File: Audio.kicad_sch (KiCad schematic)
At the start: 21 parts, among them CN2 PJ-3537S, U3 SGTL5000XNAA3R2, U8 PCM1807PW, X1 SMD-3225_4P 12.288MHZ 12PF

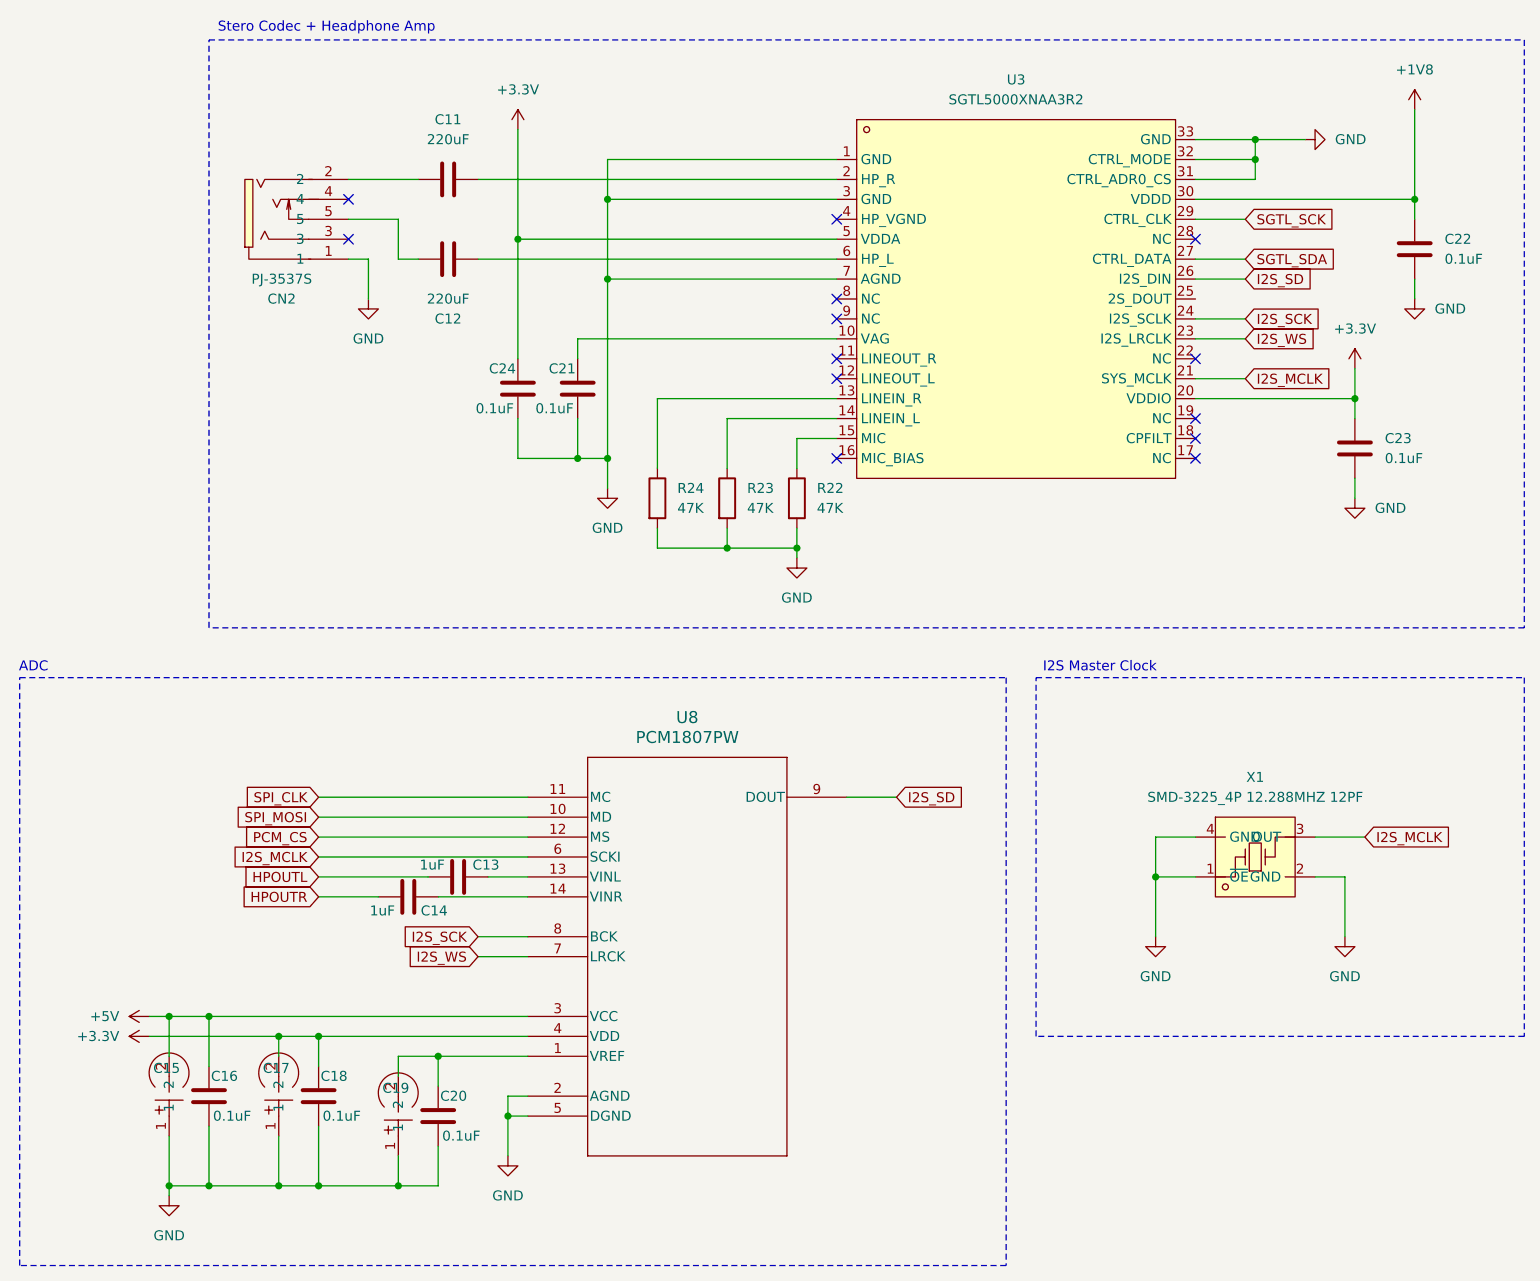
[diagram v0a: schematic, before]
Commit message: start of adding esp32 module
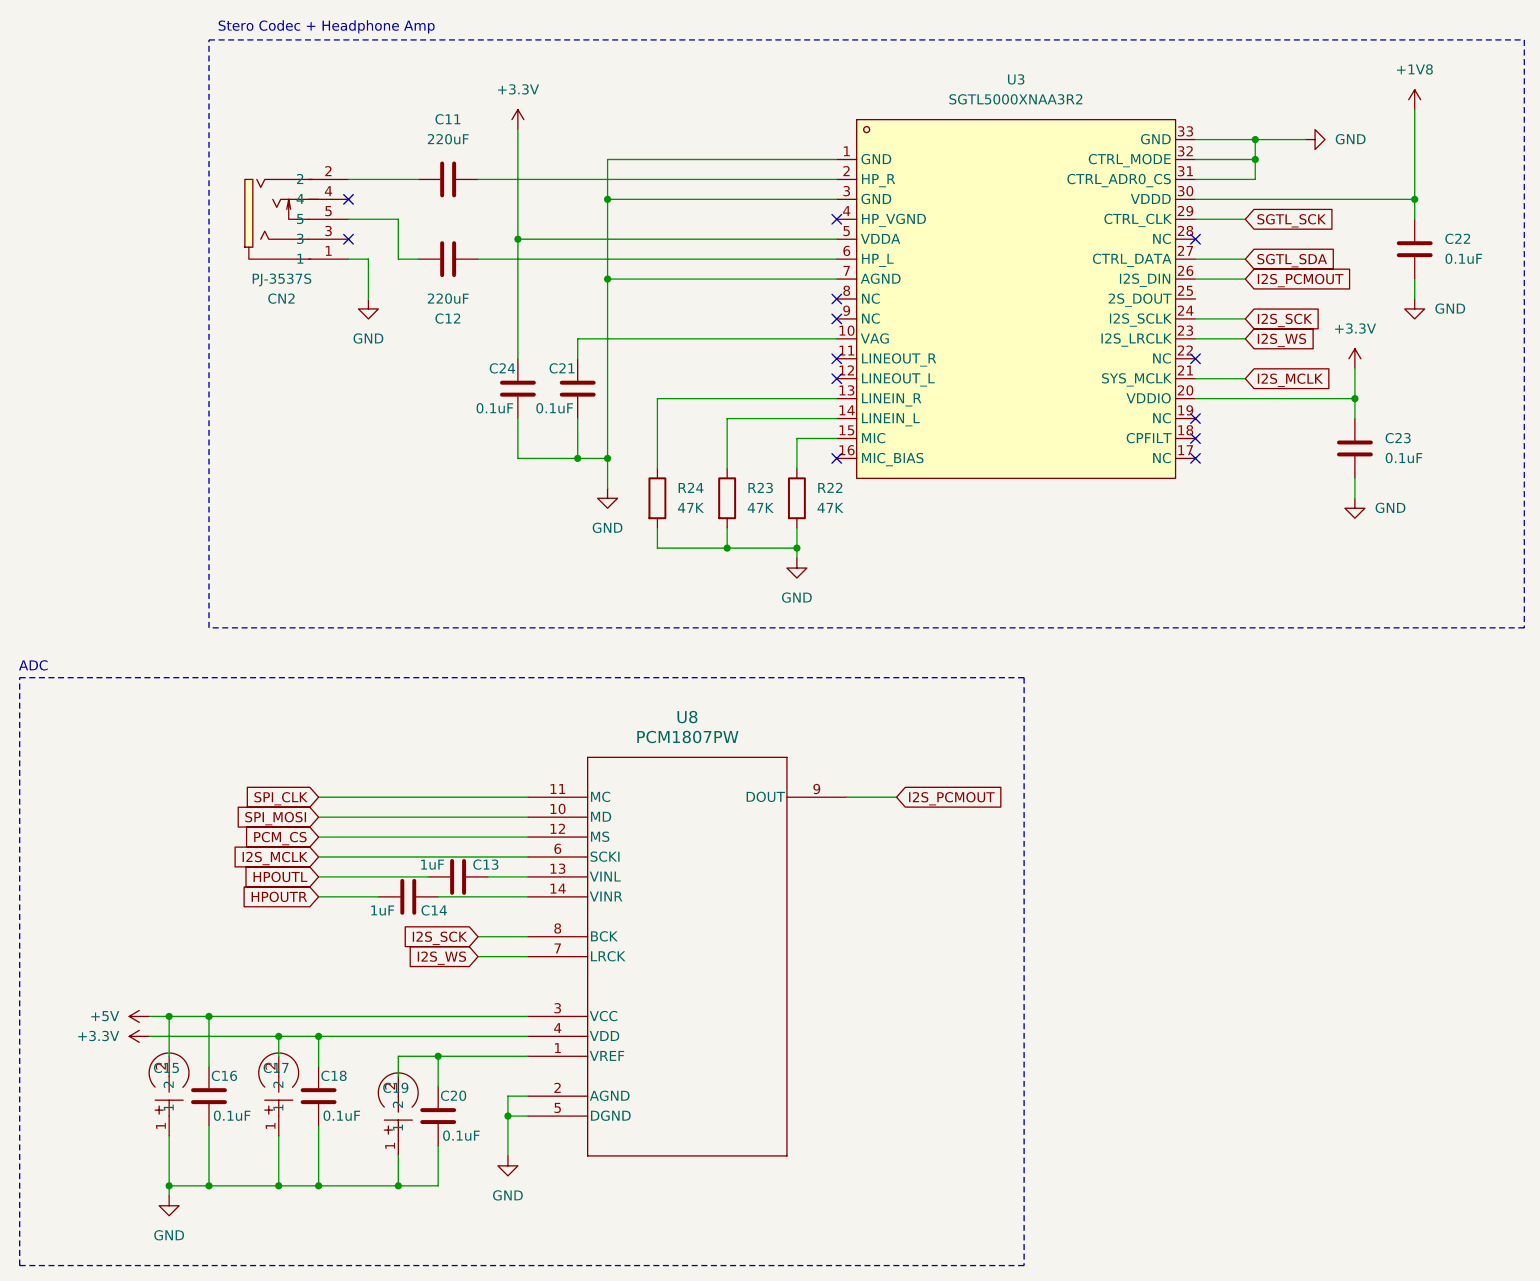
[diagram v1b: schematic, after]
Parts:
- removed X1: SMD-3225_4P 12.288MHZ 12PF, easyeda2kicad:CRYSTAL-SMD_4P-L3.2-W2.5-BL-2, symbol easyeda2kicad:SMD-3225_4P12.288MHZ12PF
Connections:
- net I2S_SD renamed I2S_PCMOUT
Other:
- note removed: "I2S Master Clock"
